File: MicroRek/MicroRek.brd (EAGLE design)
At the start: 40 x 30 mm, 18 parts, among them IC3 LSM9DS1TR

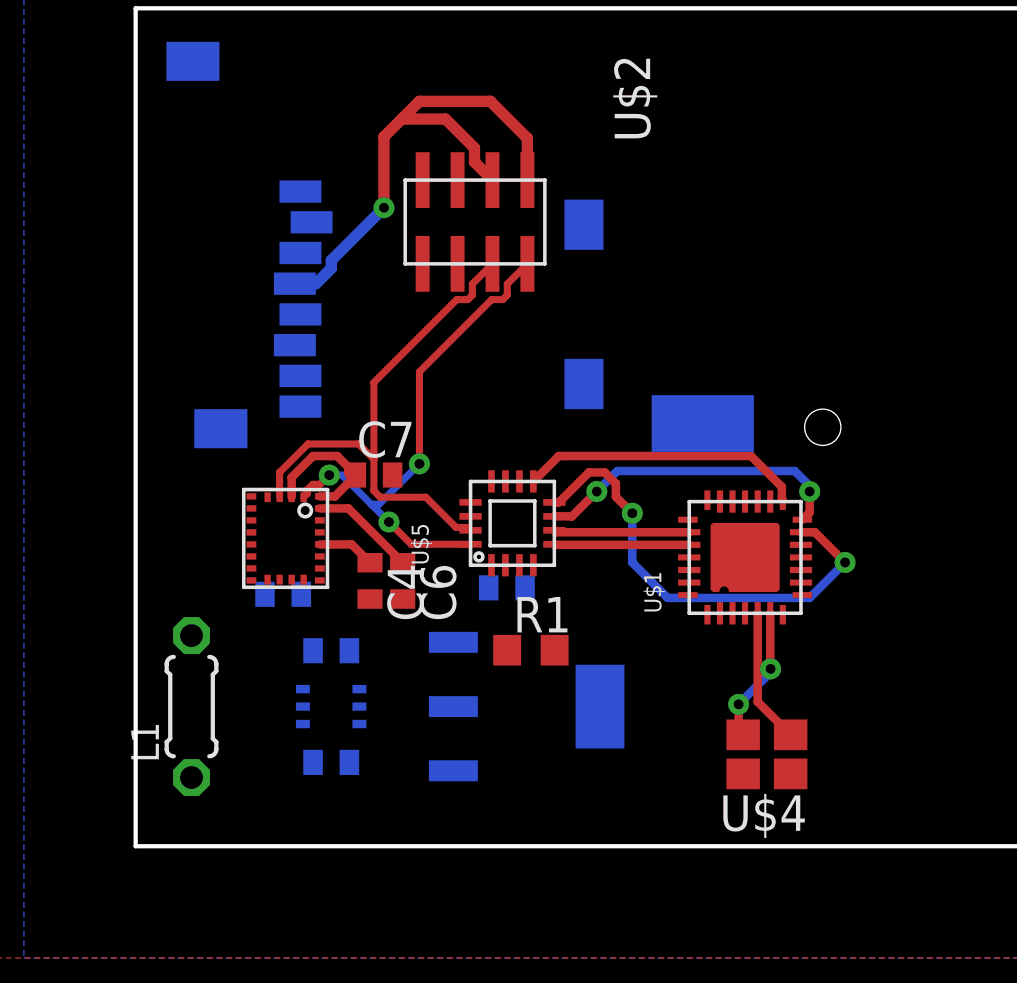
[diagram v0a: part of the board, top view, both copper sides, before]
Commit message: Updated MicroRek Board Layout
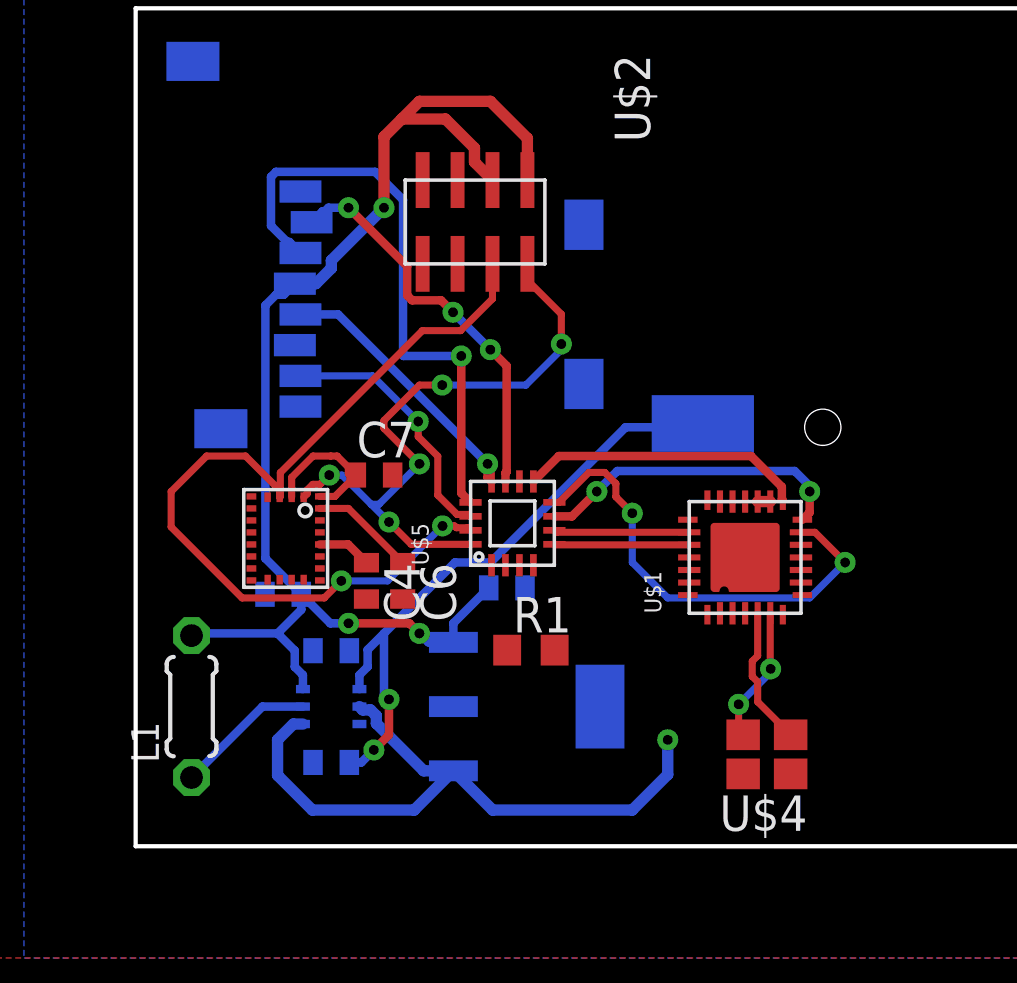
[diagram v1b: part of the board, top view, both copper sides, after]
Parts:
- moved C4 0.13 mm to (8.26, 9.50)
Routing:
- net 3.3V: track 19.2 -> 47.3 mm, vias 1 -> 3
- net 5V: track 0.00 -> 24.8 mm, vias 0 -> 1
- net N$2: track 0.00 -> 22.4 mm, vias 0 -> 2
- net MOSI3: track 0.00 -> 21.5 mm, vias 0 -> 1
- net D23: track 0.00 -> 14.3 mm, vias 0 -> 3
- net SDA3: track 19.1 -> 31.7 mm, vias 0 -> 2
- net SCK3: track 0.00 -> 9.60 mm, vias 0 -> 1
- net MISO3: track 0.00 -> 9.31 mm, vias 0 -> 1
- net N$3: track 0.00 -> 5.04 mm
- net SCL3: track 18.7 -> 22.8 mm, vias 3 -> 5
